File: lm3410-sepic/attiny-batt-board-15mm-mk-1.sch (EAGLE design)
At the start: 14 parts

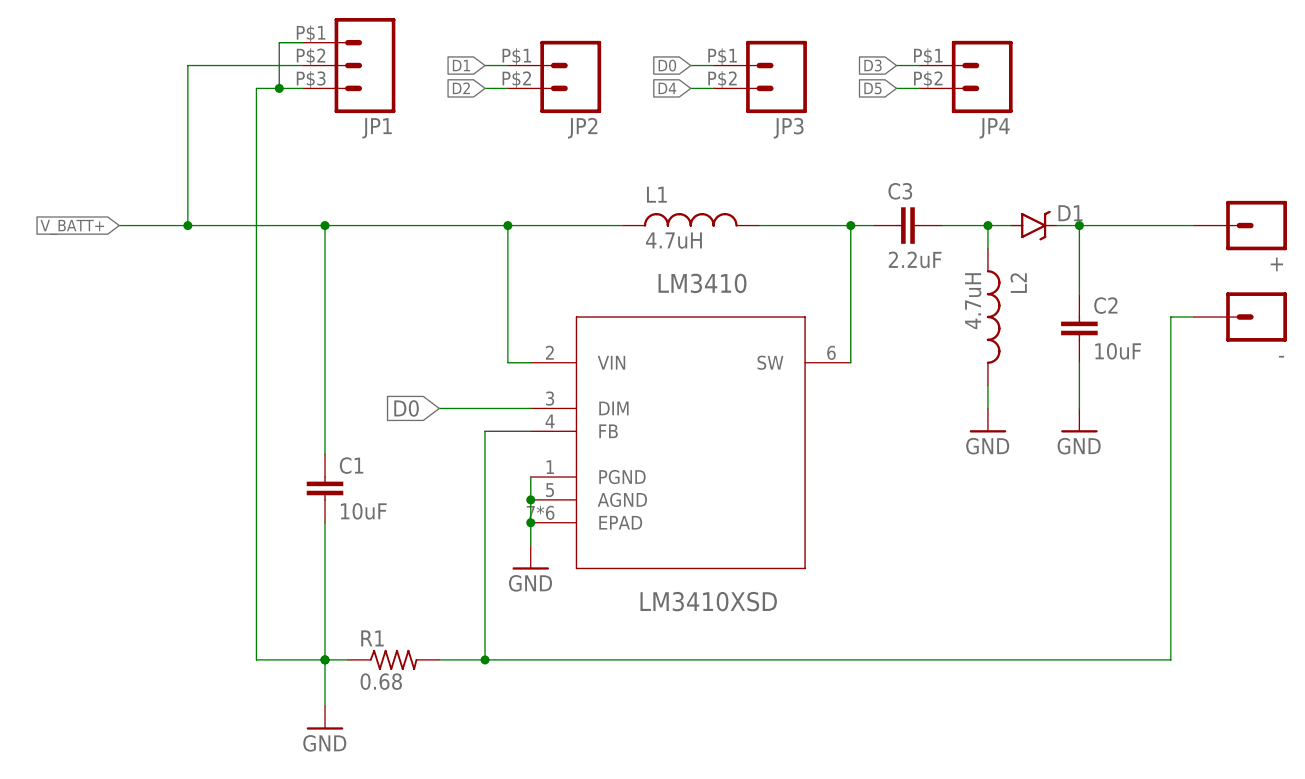
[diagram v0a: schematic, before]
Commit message: interim commit, kinda borked atm
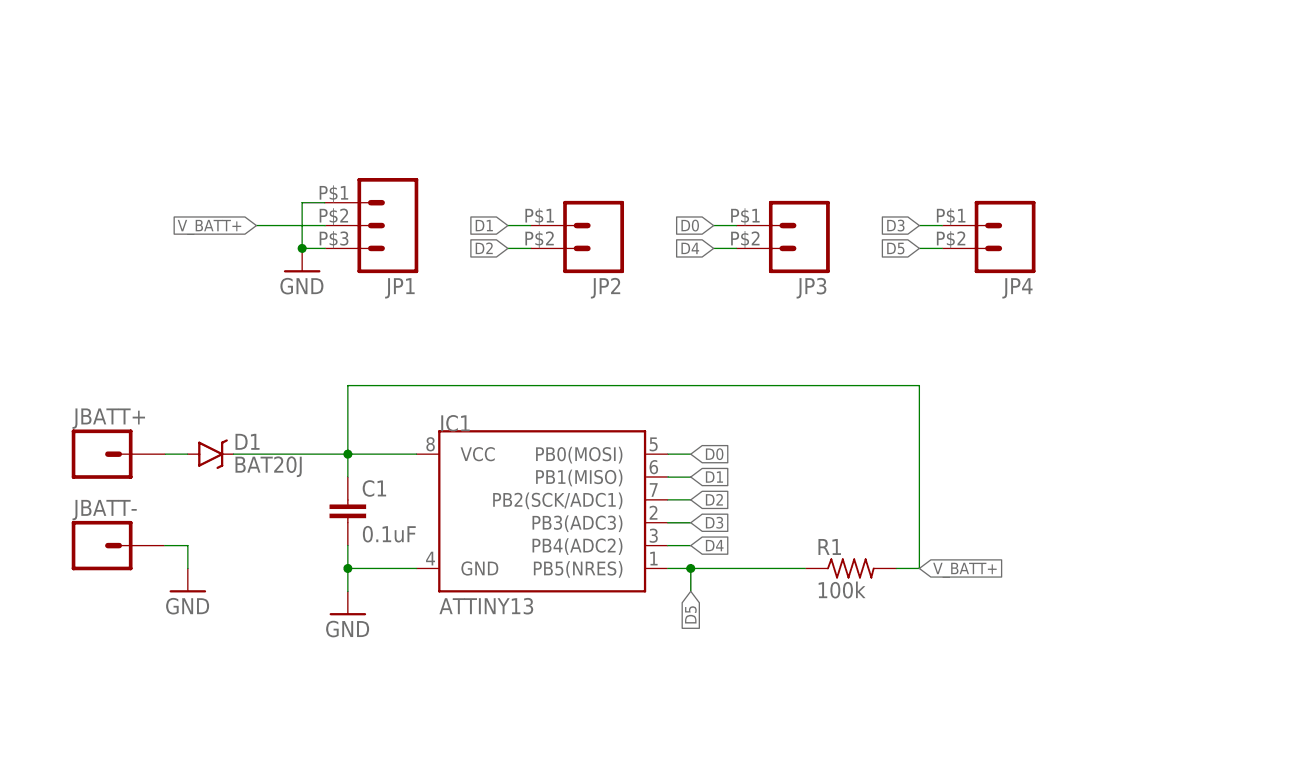
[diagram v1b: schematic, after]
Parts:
- removed +: M01PTH-KIT, A_butts:M01PTH-KIT
- removed -: M01NOSILK-KIT, A_butts:M01NOSILK-KIT
- removed C2: 10uF, A_butts:CAPACITOR-CERAMICC0603
- removed C3: 2.2uF, A_butts:CAPACITOR-CERAMICC0805
- removed L1, L2: 4.7uH, A_butts:INDUCTORIFSC-0806
- removed LM3410: LM3410XSD, A_butts:LM3410XSD
- added IC1: ATTINY13, A_butts:ATTINY13SOIC
- added JBATT+, JBATT-: M01NOT-A-VIA-NOPE, A_butts:M01NOT-A-VIA-NOPE
- C1: value 10uF -> 0.1uF
- R1: value 0.68 -> 100k; device A_butts:RESISTORR1206 -> A_butts:RESISTORR0603
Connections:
- removed net LED_ANODE: +.1, C2.1, D1.C
- removed net N$1: C3.2, D1.A, L2.1
- removed net N$6: -.1, LM3410.FB, R1.2
- removed net SW: C3.1, L1.2, LM3410.SW
- new net BATT_IN: D1.A, JBATT+.1
- net D0: now also IC1.PB0(MOSI); no longer LM3410.DIM
- net D1: now also IC1.PB1(MISO)
- net D2: now also IC1.PB2(SCK/ADC1)
- net D3: now also IC1.PB3(ADC3)
- net D4: now also IC1.PB4(ADC2)
- net D5: now also IC1.PB5(NRES), R1.1
- net GND: now also IC1.GND, JBATT-.1; no longer C2.2, L2.2, LM3410.AGND, LM3410.EPAD, LM3410.PGND, R1.1
- net V_BATT+: now also D1.C, IC1.VCC, R1.2; no longer L1.1, LM3410.VIN
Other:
- moved on the sheet: C1, D1, JP1, JP2, JP3, JP4, R1
